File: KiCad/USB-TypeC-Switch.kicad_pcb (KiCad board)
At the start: 4 copper layers, 48.5 x 50 mm, 59 parts, among them J1 USB_C_IN_1, J2 USB_C_IN_2, J3 USB_C_OUT, J4 Conn_02x05_Odd_Even, SW1 SW_Push, U1 FUSB340TMX, U2 FUSB340TMX, U3 NL3S588, U4 AP63205WU, U5 UCS3205-E_Q8A, U6 UCS3205-E_Q8A, U7 NL3S588, U8 AZ1117C-3.3, U9 ATSAMD21E15B-M

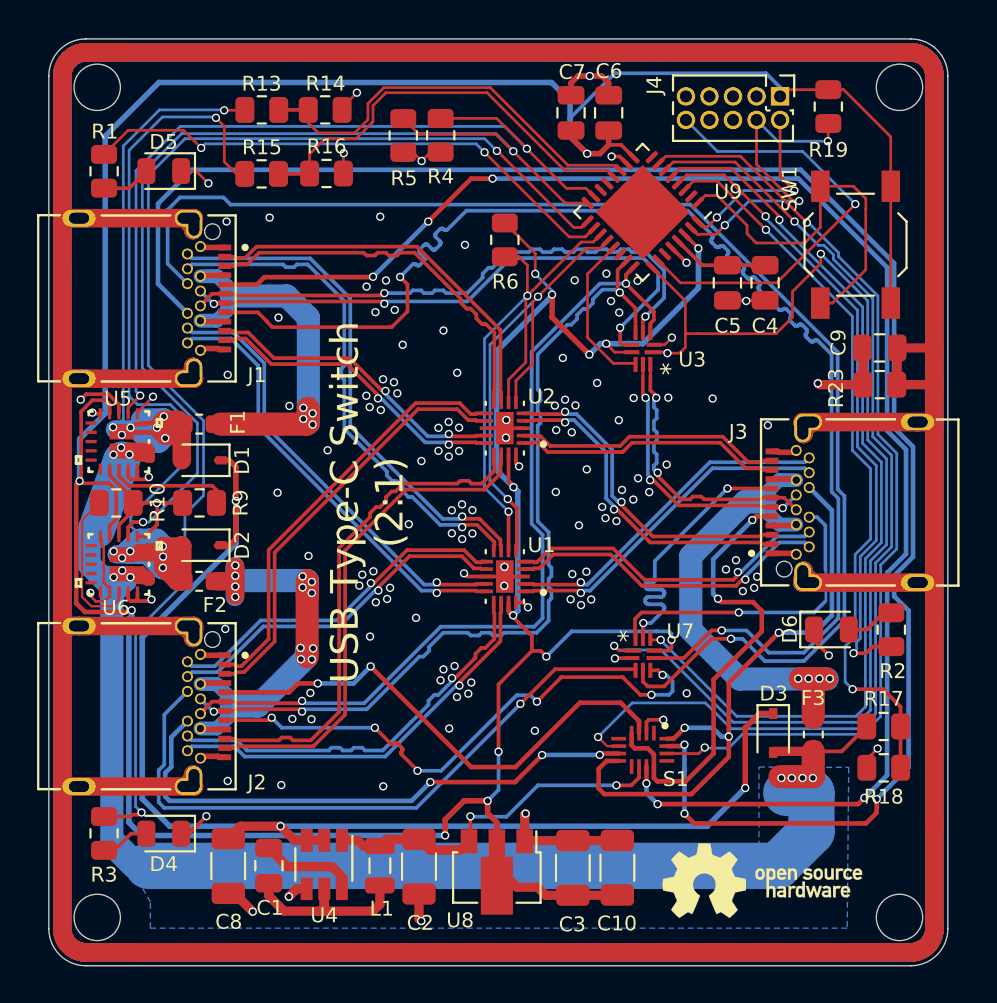
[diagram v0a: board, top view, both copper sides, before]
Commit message: Fix USB 2.0 signal polarity (+others)
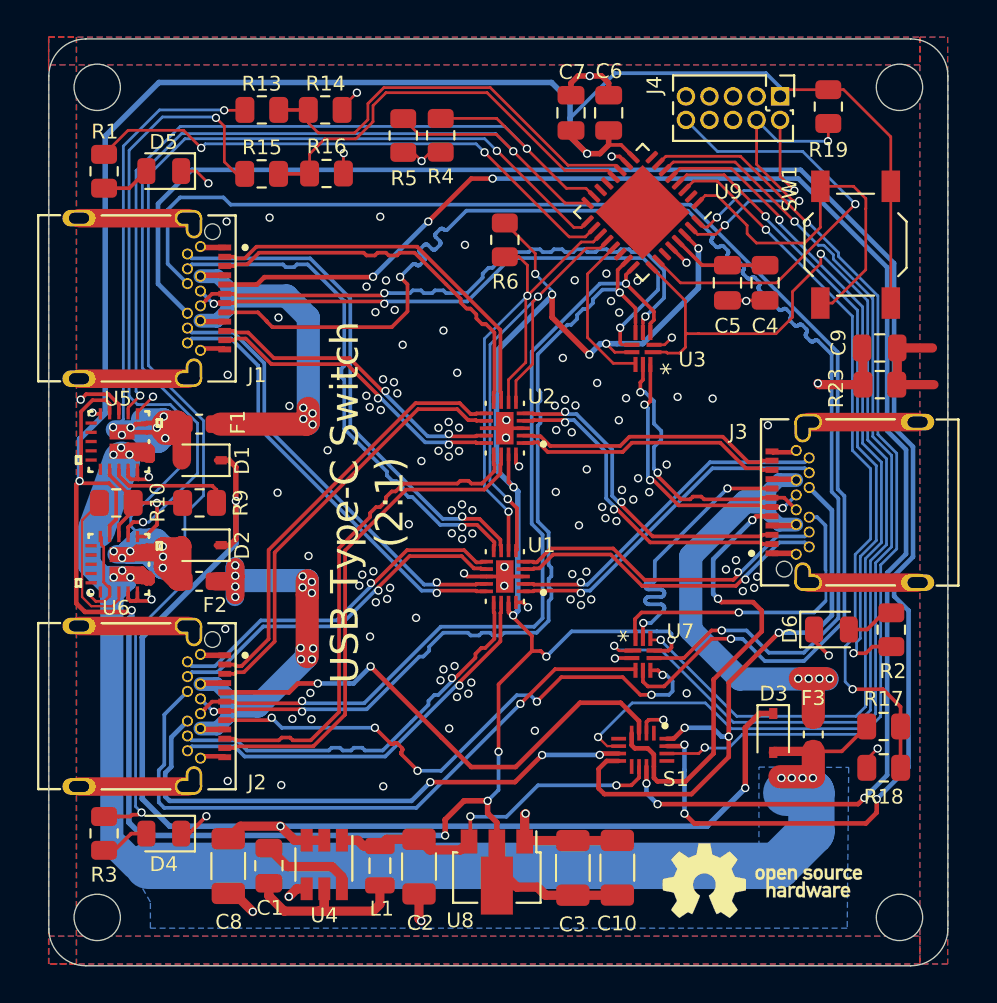
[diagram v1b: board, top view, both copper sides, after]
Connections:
- net /USB 2.0 and Misc Signal Switching/D_2_N renamed /Control/D_N_uC
- net /USB 2.0 and Misc Signal Switching/D_2_P renamed /Control/D_P_uC
- net /USB 2.0 and Misc Signal Switching/SEL renamed /Control/SEL_USB2_SBU
- net /USB 3 Signal Switching/OE_N renamed /Control/OE_N_USB3
- net /USB 3 Signal Switching/SEL renamed /Control/SEL_USB3
- J3 pad A6: /USB 2.0 and Misc Signal Switching/D_N -> /USB 2.0 and Misc Signal Switching/D_P
- J3 pad A7: /USB 2.0 and Misc Signal Switching/D_P -> /USB 2.0 and Misc Signal Switching/D_N
- J3 pad B6: /USB 2.0 and Misc Signal Switching/D_N -> /USB 2.0 and Misc Signal Switching/D_P
- J3 pad B7: /USB 2.0 and Misc Signal Switching/D_P -> /USB 2.0 and Misc Signal Switching/D_N
- J4 pad 6: (no net) -> unconnected-(J4-Pad6)
- J4 pad 8: (no net) -> unconnected-(J4-Pad8)
- S1 pad 1: (no net) -> unconnected-(S1-Pad1)
- S1 pad 13: (no net) -> unconnected-(S1-Pad13)
- S1 pad 5: (no net) -> unconnected-(S1-Pad5)
- S1 pad 9: (no net) -> unconnected-(S1-Pad9)
- U5 pad 10: (no net) -> unconnected-(U5-Pad10)
- U5 pad 11: (no net) -> unconnected-(U5-Pad11)
- U5 pad 6: (no net) -> unconnected-(U5-Pad6)
- U5 pad 7: (no net) -> unconnected-(U5-Pad7)
- U5 pad 8: (no net) -> unconnected-(U5-Pad8)
- U5 pad 9: (no net) -> unconnected-(U5-Pad9)
- U6 pad 10: (no net) -> unconnected-(U6-Pad10)
- U6 pad 11: (no net) -> unconnected-(U6-Pad11)
- U6 pad 6: (no net) -> unconnected-(U6-Pad6)
- U6 pad 7: (no net) -> unconnected-(U6-Pad7)
- U6 pad 8: (no net) -> unconnected-(U6-Pad8)
- U6 pad 9: (no net) -> unconnected-(U6-Pad9)
- U9 pad 13: (no net) -> unconnected-(U9-Pad13)
- U9 pad 14: (no net) -> unconnected-(U9-Pad14)
- U9 pad 2: (no net) -> unconnected-(U9-Pad2)
- U9 pad 22: (no net) -> unconnected-(U9-Pad22)
- U9 pad 27: (no net) -> unconnected-(U9-Pad27)
- U9 pad 33: (no net) -> unconnected-(U9-Pad33)
- U9 pad 8: (no net) -> unconnected-(U9-Pad8)
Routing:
- net GNDS: track 457.0 -> 41.3 mm
- net GND: track 77.2 -> 76.7 mm
- net /USB 2.0 and Misc Signal Switching/D_P: track 15.2 -> 15.4 mm, vias 2 -> 3
- net /USB 2.0 and Misc Signal Switching/D_N: track 15.3 -> 15.4 mm, vias 3 -> 2
- net /Control/SEL_USB2_SBU: vias 3 -> 2
- added copper zone on B.Cu, net GNDS
- added copper zone on F.Cu, net GNDS
